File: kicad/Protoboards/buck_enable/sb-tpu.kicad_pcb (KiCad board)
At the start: 6 copper layers, 43 x 43 mm, 186 parts, among them IC2 LM3370SD-4221/NOPB, IC3 G313-06329-00, IC4 NCP170ASN180T2G, IC6 74LVC2G66GT,115, IC8 SN74AUP1T34QDCKRQ1, IC9 PTN5150AHXMP, J1 DX07S016JA1R1500, J2 Conn_01x04, J3 CES-104-02-G-S, J4 CES-104-02-G-S, J5 CES-116-02-G-S, J6 CES-116-02-G-S, J7 CES-104-02-G-S, J8 CES-104-02-G-S, Q1 DMN3900UFA-7B, Q2 DMN3900UFA-7B, Q3 DMN3900UFA-7B, Q4 DMN3900UFA-7B, SW1 SKRPADE010, SW2 SKRPADE010, U1 LTC4413EDD-1_TRPBF, U2 TCR2LN33,LF(SE, U5 MT29F1G01ABBFDWB-IT_F_TR, U6 MT48H32M16LFB4-6 AAT:C TR, U7 SIP32408DNP-T1-GE4, Y1 FC-135_32.7680KA-AG3, Y2 FA-20H_24.0000MF20X-K3

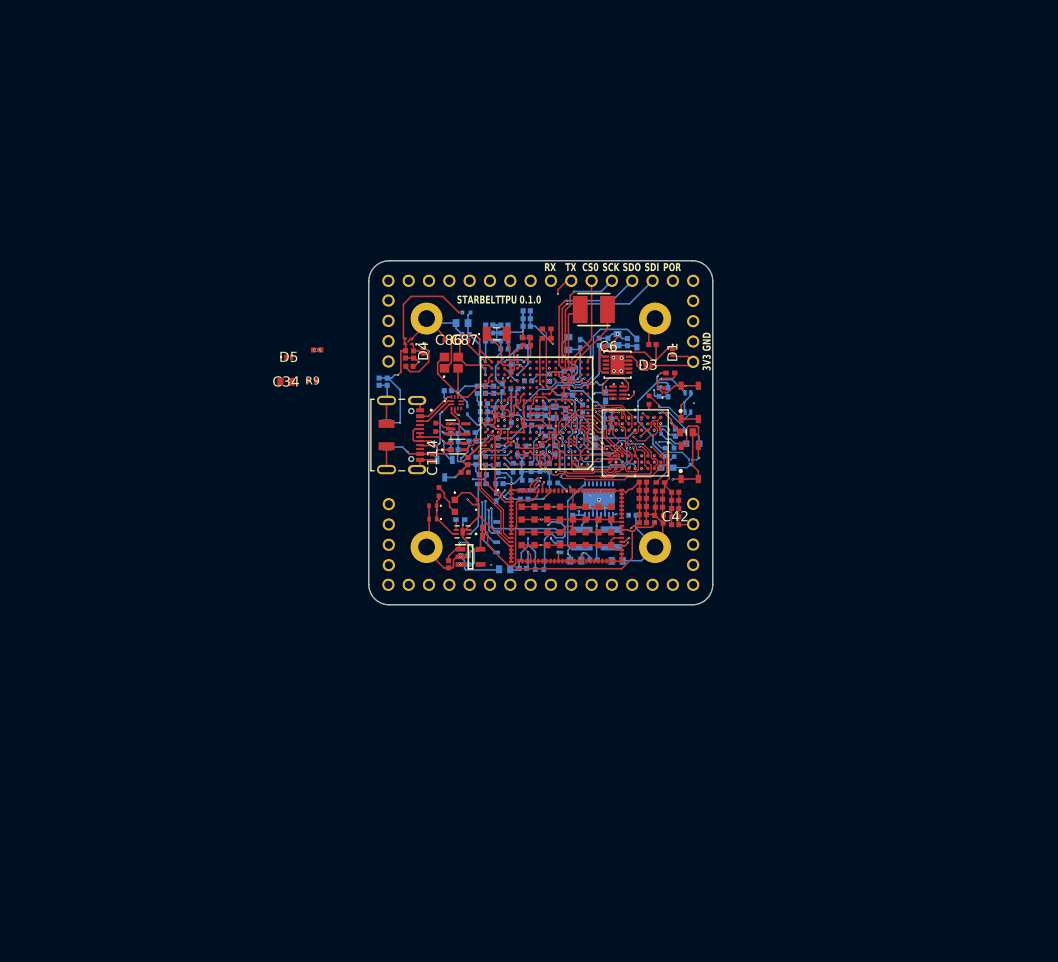
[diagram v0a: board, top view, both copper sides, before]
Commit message: [PROTOTYPES] Protoboard layout completed
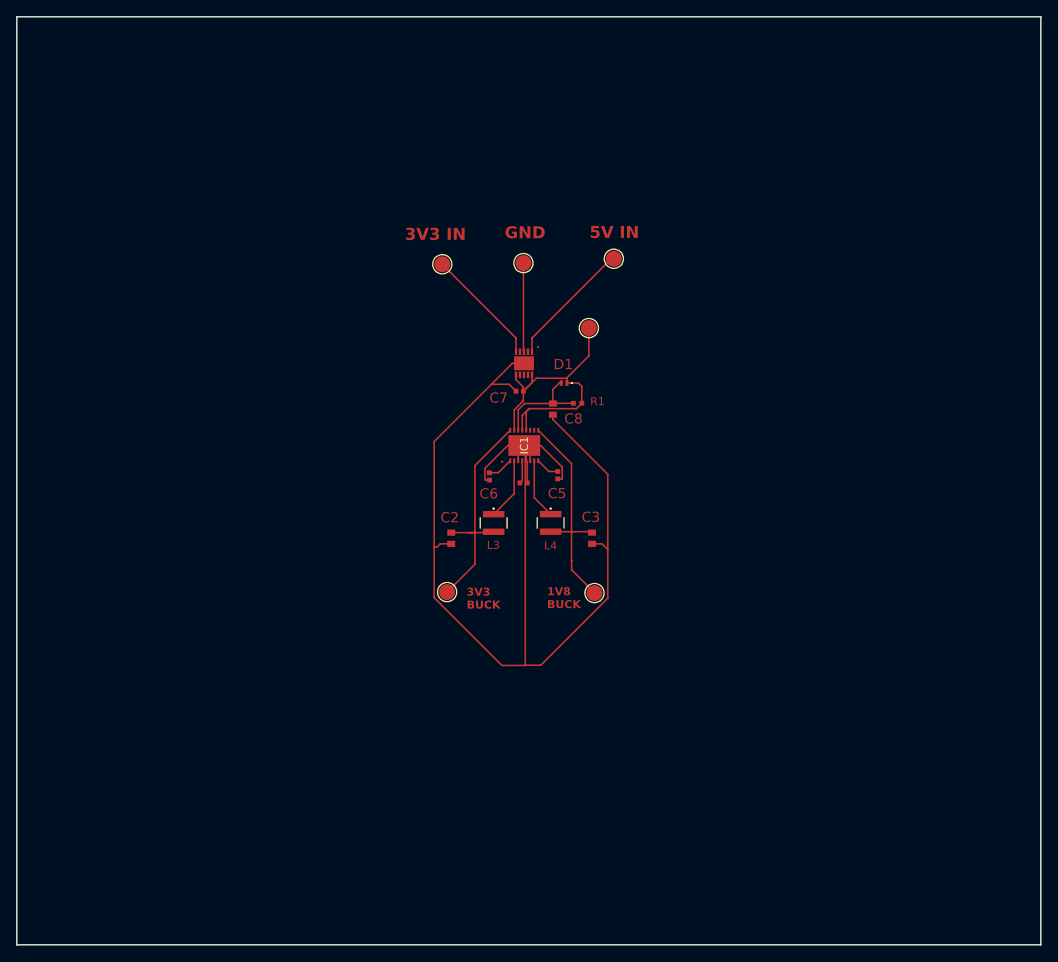
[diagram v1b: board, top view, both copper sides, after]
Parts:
- removed C1, C10, C108, C109, C110, C111, C112, C113, C57, C58, C71, C73, C85, C91: 04026D105KAT2A, footprints:CAPC1005X56N
- removed C100, C101, C102, C105, C106, C61, C74, C77, C78, C79, C90, C97, C99: CL05A225MQ5NSNC, footprints:CAPC1005X57N
- removed C103, C104, C114, C21, C22, C23, C42, C65, C66, C67, C70, C75, C76, C95, C96, C98: GRM155R60J475KE96D, footprints:CAPC1005X70N
- removed C107: GRM1555C1E100JA01D, footprints:CAPC1005X70N
- removed C11, C115, C30, C32, C33, C35, C36, C37, C38, C40, C43, C44, C45, C46, C47, C48, C49, C50, C51, C52, C53, C54, C55, C56, C63, C68, C69, C82, C88, C89, C92, C93, C94: 04023C104JAT2A, footprints:CAPC1005X56N
- removed C16, C17, C80, C81: 0603ZW106MAT2A, footprints:CAPC1608X90N
- removed C34, C39: 06036D105MAT2A, footprints:CAPC1608X90N
- removed C41, C62, C64, C83, C84: 04026D226MAT2A, footprints:CAPC1005X56N
- removed C59, C60: GRM158R61A226ME15D, footprints:GRM15x
- removed C72: JMK105BJ224KV-F, footprints:cap_UMK105 CG080CV-F_TAY
- removed C86, C87: GRM1555C1H160JA01D, footprints:CAPC1005X70N
- removed D10: LTST-C190AKT, footprints:LEDM1608X80
- removed D11: APG1608ZGCK, footprints:LED_APG1608ZGCK
- removed D2: RBS2MM40CTR, footprints:RBS2MM40CTR
- removed D3, D4, D5, D7, D8: CDBQC0240L-HF, footprints:CDBQC0240LHF
- removed D6: ESD9R3.3ST5G, footprints:SODFL1006X40N
- removed D9: PESD5V0S2BT,215, footprints:SOT95P230X110-3N
- removed FL1: DLW21HN900SQ2L, footprints:FIL_DLW21HN900SQ2L
- removed IC2: LM3370SD-4221/NOPB, footprints:SDA16B
- removed IC3: G313-06329-00, footprints:G3130632900
- removed IC4: NCP170ASN180T2G, footprints:SOT95P275X110-5N
- removed IC6: 74LVC2G66GT,115, footprints:74AVC9112GTX
- removed IC8: SN74AUP1T34QDCKRQ1, footprints:SOT65P210X110-5N
- removed IC9: PTN5150AHXMP, footprints:PTN5150AHXMP
- removed J1: DX07S016JA1R1500, footprints:JAE_DX07S016JA1R1500
- removed J2: Conn_01x04, footprints:SB_Stack_Mounting_Holes
- removed J3, J4, J7, J8: CES-104-02-G-S, footprints:CES-104-XX-Y-S
- removed J5, J6: CES-116-02-G-S, footprints:CES-116-XX-Y-S
- removed L1, L2: NR3010T2R2M, footprints:IND_TAIYO_NR3010_TAY
- removed L10, L11, L5, L7, L8, L9: BLM15AG121SN1D, footprints:IND_BLM15_0402_MUR
- removed L6: 74404041047, footprints:INDPM4040X120N
- removed LED1: LTW-C193TS5, footprints:LTWC193TS5
- removed Q1, Q2, Q3, Q4: DMN3900UFA-7B, footprints:DMN3900UFA7B
- removed R11, R13, R15, R18, R20, R22, R28, R30, R34, R9: CRCW040247K0FKTD, footprints:CRCW0402200KFKED
- removed R16, R35, R36, R37: CRCW040210K0FKEE, footprints:CRCW0402200KFKED
- removed R23, R25, R31, R38, R43, R55, R56: 0402WGF4701TCE, footprints:RESC1005X40N
- removed R39, R41, R42, R45, R46: RCWE0402R100JNEA, footprints:RESC1006X45N
- removed R40, R57, R59, R60: CRCW0402100RFKEE, footprints:CRCW0402200KFKED
- removed R44: MCT06030C3002FP500, footprints:RESC1608X55N
- removed R47: ERJPA2J105X, footprints:RES_ERJPA2J105X
- removed R48: CRCW0603430KJNEA, footprints:RESC1608X50N
- removed R50, R51: CRCW04022K20FKEDHP, footprints:RESC1005X40N
- removed R52, R54, R58: CRCW0402100KJNED, footprints:CRCW0402200KFKED
- removed R7: MCT06030E1002BP500, footprints:RESC1608X55N
- removed SW1, SW2: SKRPADE010, footprints:SKRPADE010_AAL
- removed U1: LTC4413EDD-1_TRPBF, footprints:DFN-10_DD
- removed U3: ~, footprints:BGA289C80P17X17_1400X1400X152
- removed U5: MT29F1G01ABBFDWB-IT_F_TR, footprints:SON127P800X600X65-8N
- removed U6: MT48H32M16LFB4-6 AAT:C TR, footprints:VFBGA54_8X8_MRN
- removed U7: SIP32408DNP-T1-GE4, footprints:TDFN_8DNP-T1-GE4_VIS
- removed Y1: FC-135_32.7680KA-AG3, footprints:FC135327680KAAG3
- removed Y2: FA-20H_24.0000MF20X-K3, footprints:FA20H160000MF12ZAC3
- added C2: 0603ZW106MAT2A, footprints:CAPC1608X90N, F.Cu at (130.3, 114.7)
- added C3: 0603ZW106MAT2A, footprints:CAPC1608X90N, F.Cu at (147.9, 114.7)
- added C4: GRM155R60J475KE96D, footprints:CAPC1005X70N, F.Cu at (139.4, 107.8)
- added IC1: LM3370SD-4221/NOPB, footprints:SDA16B, F.Cu at (139.4, 103.1)
- added L3: NR3010T2R2M, footprints:IND_TAIYO_NR3010_TAY, F.Cu at (135.6, 112.8)
- added L4: NR3010T2R2M, footprints:IND_TAIYO_NR3010_TAY, F.Cu at (142.7, 112.8)
- added R1: CRCW040247K0FKTD, footprints:CRCW0402200KFKED, F.Cu at (146.1, 97.8)
- added REF**: TestPoint_Pad_D2.0mm, TestPoint:TestPoint_Pad_D2.0mm, F.Cu at (139.3, 80.3)
- added TP1: TestPoint, TestPoint:TestPoint_Pad_D2.0mm, F.Cu at (129.2, 80.4)
- added TP2: TestPoint, TestPoint:TestPoint_Pad_D2.0mm, F.Cu at (150.6, 79.7)
- added TP4: TestPoint, TestPoint:TestPoint_Pad_D2.0mm, F.Cu at (129.8, 121.4)
- added TP6: TestPoint, TestPoint:TestPoint_Pad_D2.0mm, F.Cu at (148.2, 121.5)
- added TP7: TestPoint, TestPoint:TestPoint_Pad_D2.0mm, F.Cu at (147.5, 88.4)
- C5, C7: value 04026D105KAT2A -> GRM155R60J475KE96D; footprint footprints:CAPC1005X56N -> footprints:CAPC1005X70N
- C8: value CL05A225MQ5NSNC -> 06036D105MAT2A; footprint footprints:CAPC1005X57N -> footprints:CAPC1608X90N
- U2: value TCR2LN33,LF(SE -> LTC4413EDD-1_TRPBF; footprint footprints:VREG_TCR2LN33 -> footprints:DFN-10_DD
- moved C5 23.5 mm to (143.6, 106.8)
- moved C6 22.0 mm to (135.1, 107.0), turned to -90 degrees
- moved U2 14.7 mm to (139.4, 92.8), turned to -90 degrees
- moved C7 14.1 mm to (138.9, 96.3), turned to 180 degrees
- moved D1 14.1 mm to (144.4, 95.3), turned to 180 degrees
- moved C8 9.23 mm to (143.0, 98.5), turned to -90 degrees
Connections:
- C5 pad 1: Net-(D4-A) -> VSYS
- C6 pad 1: VDD_3V3 -> VSYS
- C7 pad 1: VSYS_3V3 -> VSYS
- C8 pad 1: VDD_SNVS_DIG -> Net-(D1-A)
- D1 pad 1: VDD_3V3 -> VSYS
- D1 pad 2: +3V3 -> Net-(D1-A)
- U2 pad 1: Net-(D4-A) -> VSYS_DA
- U2 pad 3: VSYS -> GND
- U2 pad 4: VSYS -> GND
- U2 pad 5: GND -> +3V3
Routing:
- net GND: track 371.2 -> 161.1 mm, vias 51 -> 0
- net VDD_1V8: track 171.3 -> 28.1 mm, vias 17 -> 0
- net VDD_3V3: track 106.2 -> 0.00 mm, vias 6 -> 0
- net MCM_1V8: track 85.6 -> 0.00 mm, vias 3 -> 0
- net MCM_3V3: track 80.3 -> 0.00 mm, vias 6 -> 0
- net POR_B: track 62.1 -> 0.00 mm, vias 3 -> 0
- net I2C5_SCL_MCM: track 46.2 -> 0.00 mm, vias 2 -> 0
- net VSYS_3V3: track 38.2 -> 0.00 mm, vias 3 -> 0
- net DCDC_1V8_OUT: track 37.7 -> 0.00 mm, vias 2 -> 0
- net VDD_SOC_IN: track 36.4 -> 0.00 mm, vias 2 -> 0
- net VDD_SNVS_ANA: track 36.2 -> 0.00 mm, vias 3 -> 0
- net I2C5_SCL: track 35.5 -> 0.00 mm, vias 2 -> 0
- net ADC_1V8_IN: track 34.4 -> 0.00 mm, vias 2 -> 0
- net SDRAM_1V8: track 33.0 -> 0.00 mm, vias 5 -> 0
- net VSYS: track 83.1 -> 50.5 mm, vias 8 -> 0
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- added copper zone on In1.Cu, net (none)
- removed copper zone on In1.Cu, net GND
- removed copper zone on In4.Cu, net GND
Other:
- board size 43 x 43 mm -> 128 x 116 mm
- board text added: "${REFERENCE}"
- board text added: "1V8 BUCK"
- board text added: "3V3 BUCK"
- board text added: "3V3 IN"
- board text added: "5V IN"
- board text removed: "0.1.0"
- board text removed: "3V3"
- board text removed: "CS0"
- board text removed: "POR"
- board text removed: "RX"
- board text removed: "SCK"
- board text removed: "SDI"
- board text removed: "SDO"
- board text removed: "STARBELT"
- board text removed: "TPU"
- board text removed: "TX"
